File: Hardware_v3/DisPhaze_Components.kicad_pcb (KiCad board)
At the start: 2 copper layers, 60 x 110 mm, 89 parts, among them J1 SWD_Header, J2 USB_B_Micro, J3 PItch_In, J4 PD1_Amt_In, J5 PD2_Amt_In, J6 VCA_In, J7 DAC1_Out, J8 DAC2_Out, J9 Eurorack_16_pin_power, Q1 MMBT3904, Q2 MMBT3904, SW1 Octave_Switch, SW2 DAC1_RingMod_Switch, SW3 DAC2_Mix_Switch, SW4 SW_Push, U1 STM32F405RGTx, U2 TL072, U3 MCP6004, U4 LM1117-3.3, U7 LM4040DBZ-5, Y1 12MHz_18pF

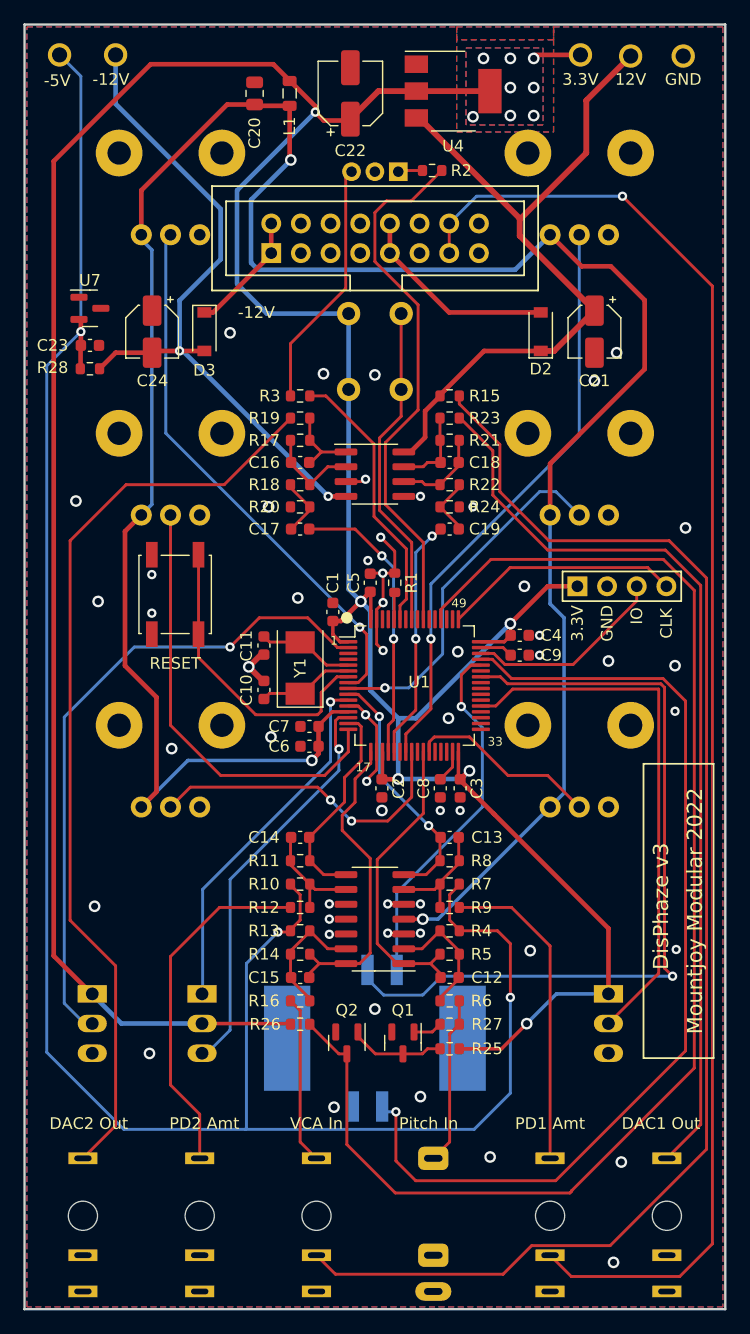
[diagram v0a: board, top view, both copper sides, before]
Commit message: More handling for MIDI issues
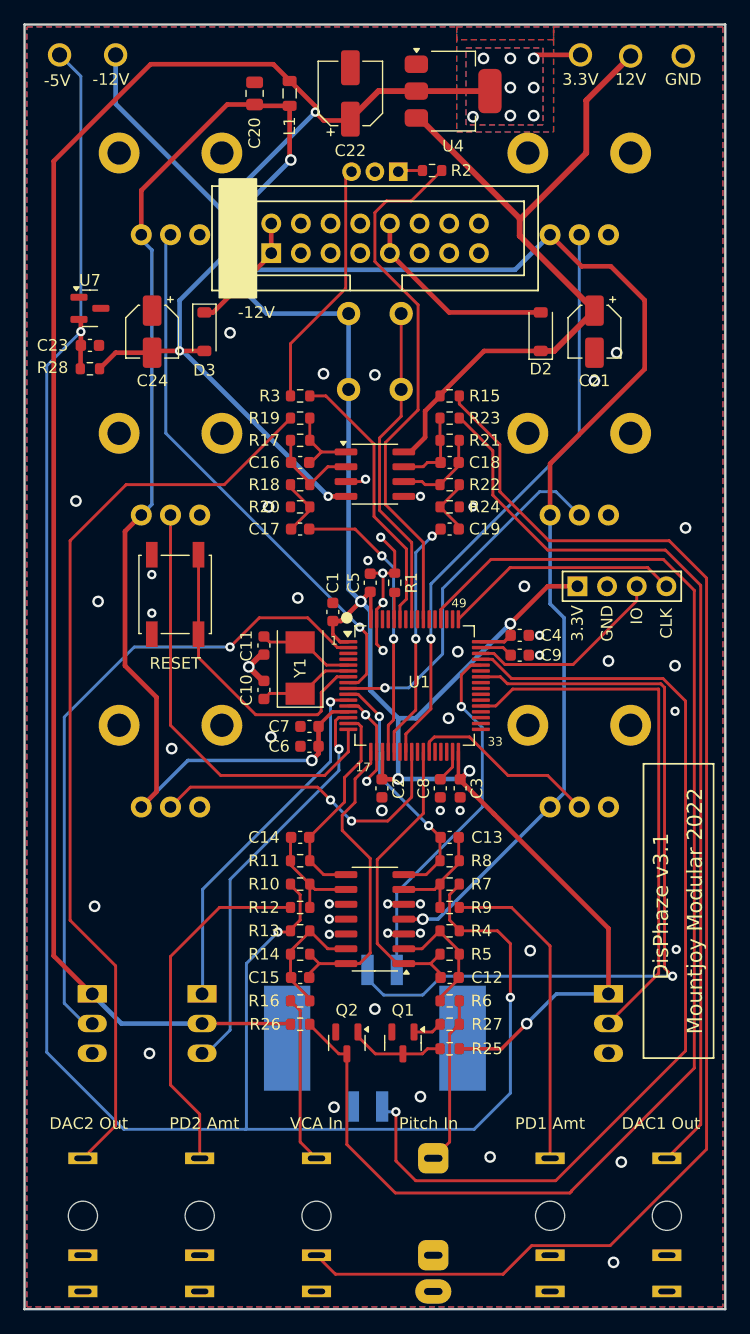
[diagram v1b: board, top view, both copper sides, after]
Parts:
- C16: value 22pF -> 1nF
- C18: value 22pF -> 1nf
- R17, R21: value 68k -> 10k
- R18, R22: value 6.8k -> 2k
- R4: value 91k -> 82k
- R5: value 56k -> 47k
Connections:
- J4 pad 2: /CV_IN -> GND
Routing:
- net /CV_IN: track 126.4 -> 0.00 mm, vias 1 -> 0
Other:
- board text added: "DisPhaze v3.1"
- board text removed: "DisPhaze v3"

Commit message: Fixed pd1 not responding in mono mode
Split original v3 schematics
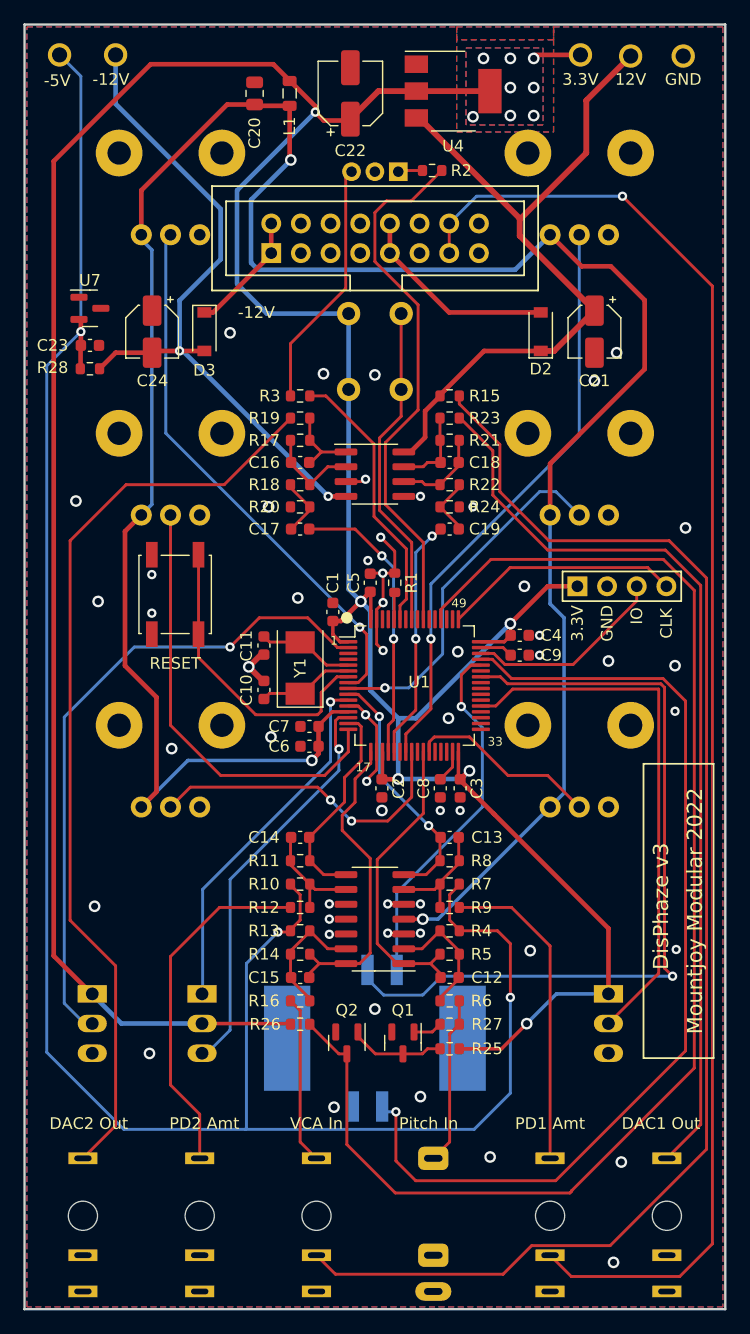
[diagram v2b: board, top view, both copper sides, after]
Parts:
- C16: value 1nF -> 22pF
- C18: value 1nf -> 22pF
- R17, R21: value 10k -> 68k
- R18, R22: value 2k -> 6.8k
- R4: value 82k -> 91k
- R5: value 47k -> 56k
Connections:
- J4 pad 2: GND -> /CV_IN
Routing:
- net /CV_IN: track 0.00 -> 126.4 mm, vias 0 -> 1
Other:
- board text added: "DisPhaze v3"
- board text removed: "DisPhaze v3.1"
